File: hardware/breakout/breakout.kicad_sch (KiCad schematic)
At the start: 81 parts, among them J1 Barrel_Jack_Switch, J2 Conn_02x40_Odd_Even, J3 Conn_02x18_Odd_Even, SW1 RESET, U1 74AHC74, U10 74AHCT245, U11 74AHC573, U12 74AHC32, U13 74AHC02, U14 74HC74, U15 74AC10, U16 DS1035-10, U2 74AHC00, U3 74AC112, U4 W65C816SxP, U5 74AHC32, U6 74AHC32, U7 74AHC125, U8 DS1813-5, U9 74HC74, X1 8MHz

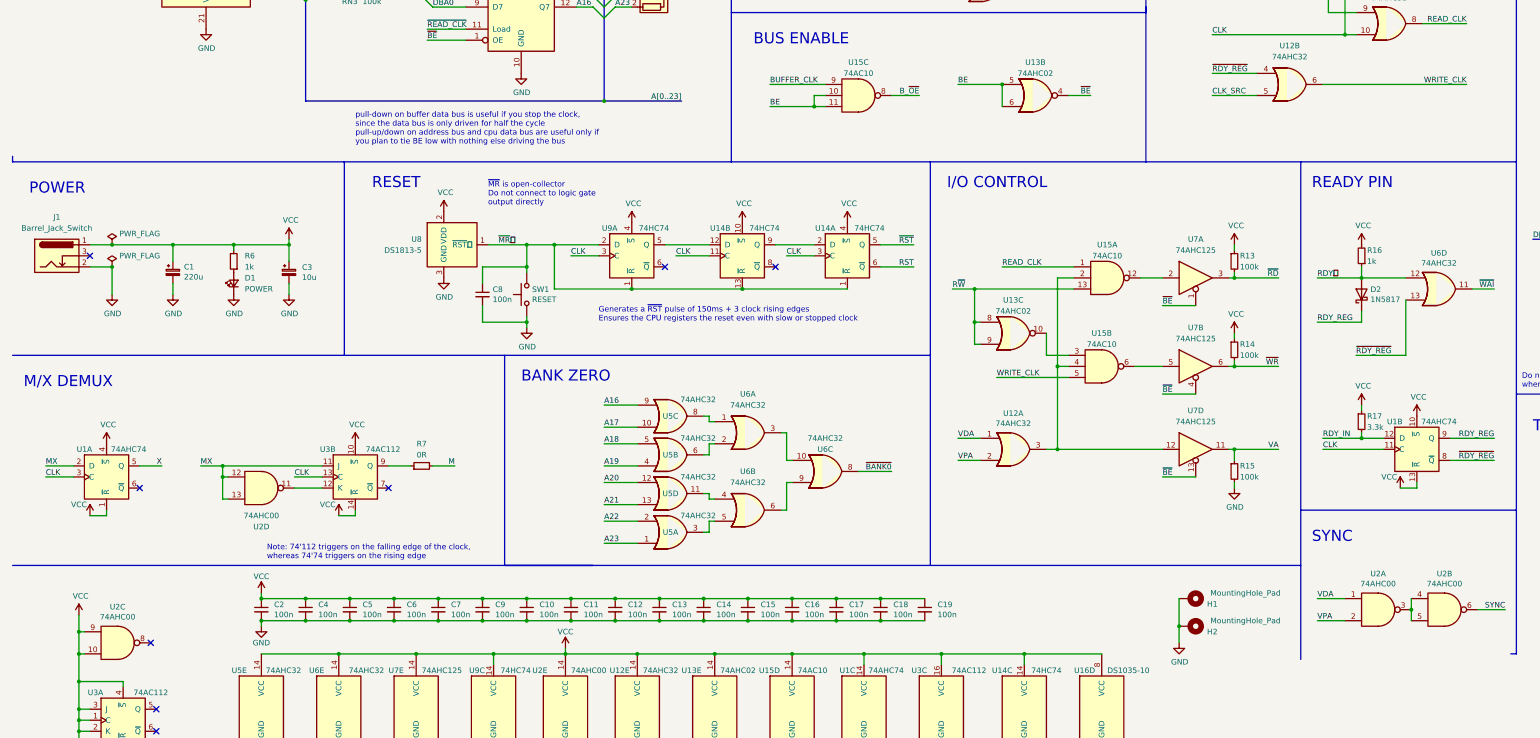
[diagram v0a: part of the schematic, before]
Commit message: Kicad 7
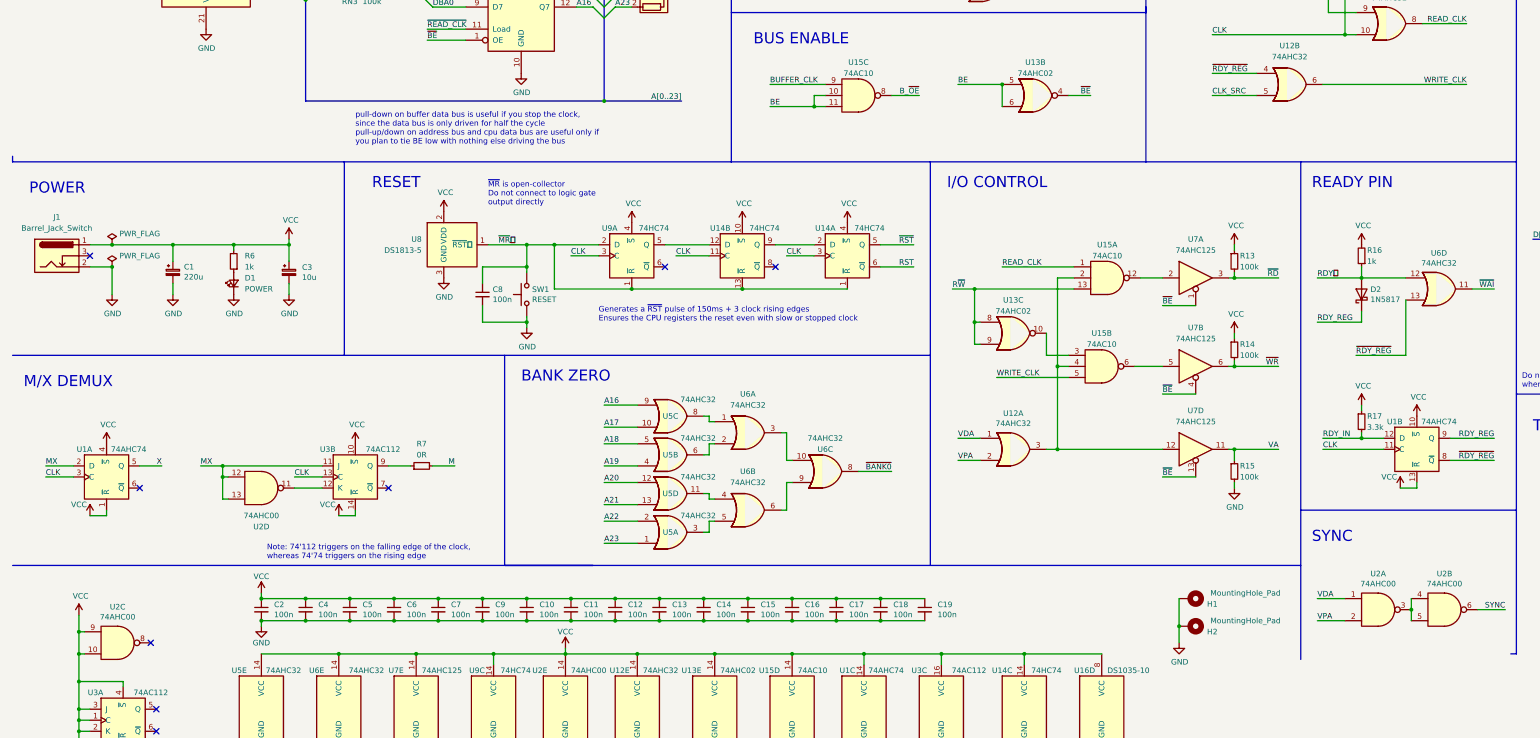
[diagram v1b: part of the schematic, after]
